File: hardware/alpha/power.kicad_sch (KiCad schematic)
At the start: 47 parts, among them J1 EXT POWER, J10 HOLE, J11 HOLE, J12 HOLE, J13 HOLE, J14 HOLE, J15 HOLE, P20 P20, P28 P28, Q3 IRLML2244, U11 TPS63700DRCT, U13 L78L05_SO8, U14 L79L05_SO8, U2 TPS61170DRVR, U6 TLE2082

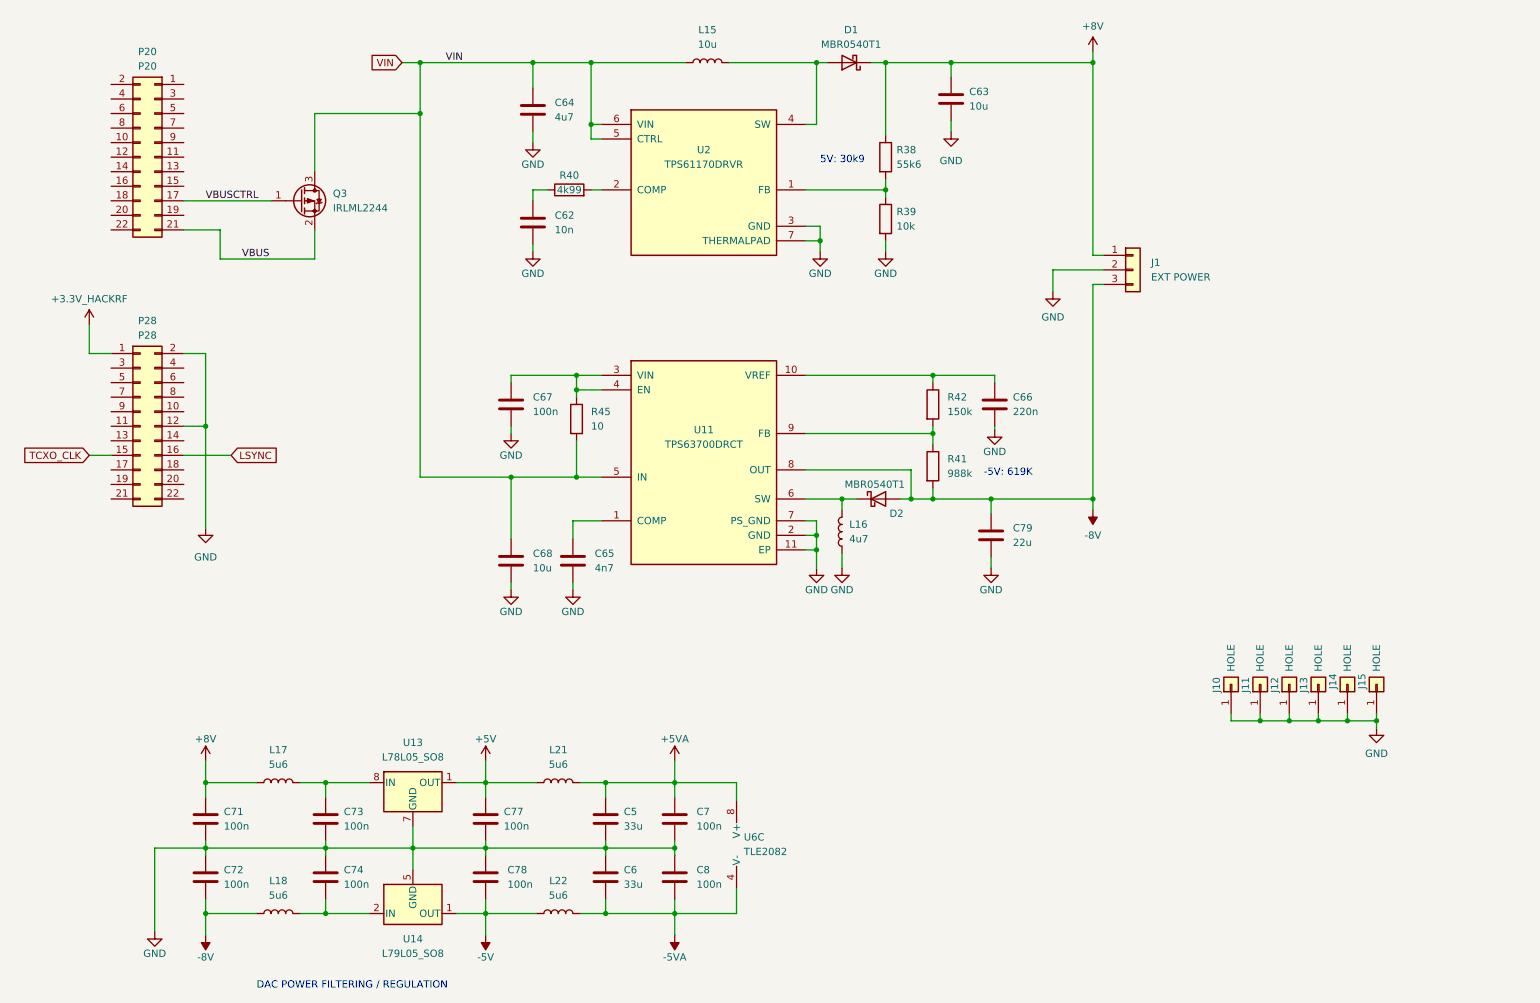
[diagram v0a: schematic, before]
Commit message: WIP
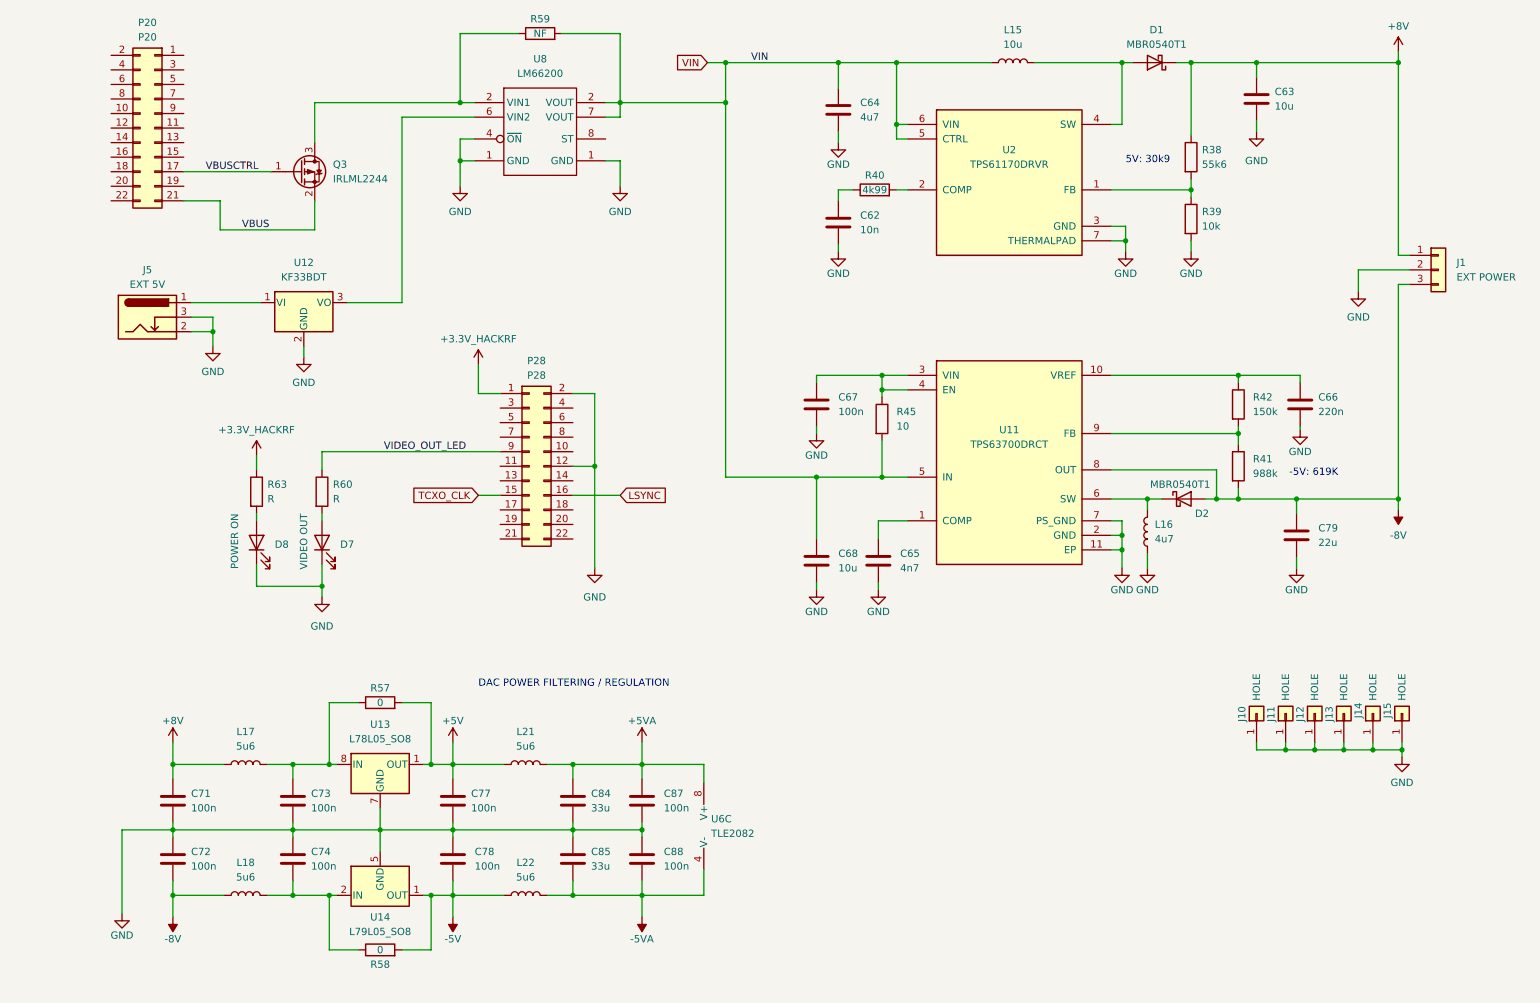
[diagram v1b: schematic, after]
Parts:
- added D7: VIDEO OUT, symbol Device:LED
- added D8: POWER ON, symbol Device:LED
- added J5: EXT 5V, symbol Connector:Barrel_Jack_Switch
- added R57, R58: 0, symbol Device:R
- added R59: NF, symbol Device:R
- added R60, R63: R, symbol Device:R
- added U12: KF33BDT, Package_TO_SOT_SMD:TO-252-2, symbol Regulator_Linear:KF33BDT
- added U8: LM66200, symbol LM66200:LM66200
- renumbered C5 to C84, C6 to C85, C7 to C87, C8 to C88
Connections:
- net +3.3V_HACKRF: now also R63.1
- net +5V: now also R57.2
- net -5V: now also R58.2
- net GND: now also D7.1 (K), D8.1 (K), J5.2, J5.3, U12.2 (GND), U8.1 (GND), U8.4 (~{ON})
- net VIN: now also R59.2, U8.2 (VOUT), U8.7 (VOUT); no longer Q3.3 (D)
- net at C74.2, L18.2, U14.2 (IN)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: now also R58.1
- net at C73.1, L17.2, U13.8 (IN): now also R57.1
- net VIDEO_OUT_LED: now reaches P28.9 (Pin_9)
- net VIDEO_OUT_LED: now also R60.1
- new net: D7.2 (A), R60.2
- new net: Q3.3 (D), R59.1, U8.2 (VOUT)
- new net: D8.2 (A), R63.2
- new net: J5.1, U12.1 (VI)
- new net: U12.3 (VO), U8.6 (VIN2)
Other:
- moved on the sheet: C62, C63, C64, C65, C66, C67, C68, C71, C72, C73, C74, C77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
